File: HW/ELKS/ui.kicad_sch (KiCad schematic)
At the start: 29 parts, among them SW1 SW, SW2 SW, SW3 SW

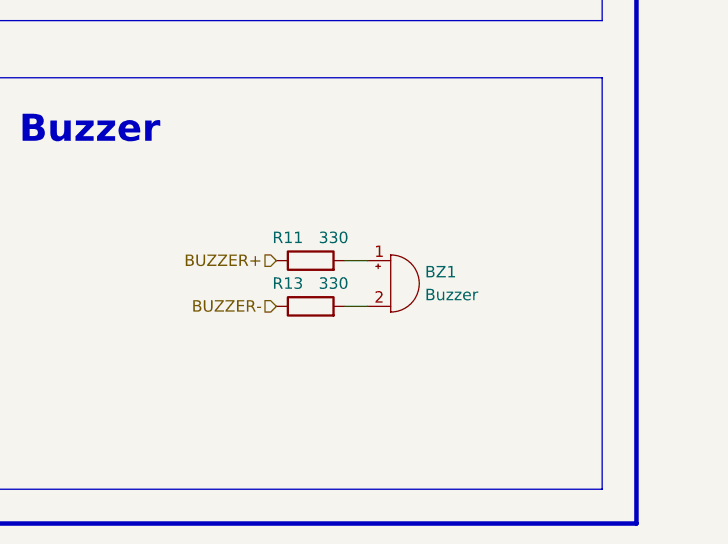
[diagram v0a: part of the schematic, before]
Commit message: Cleaning files
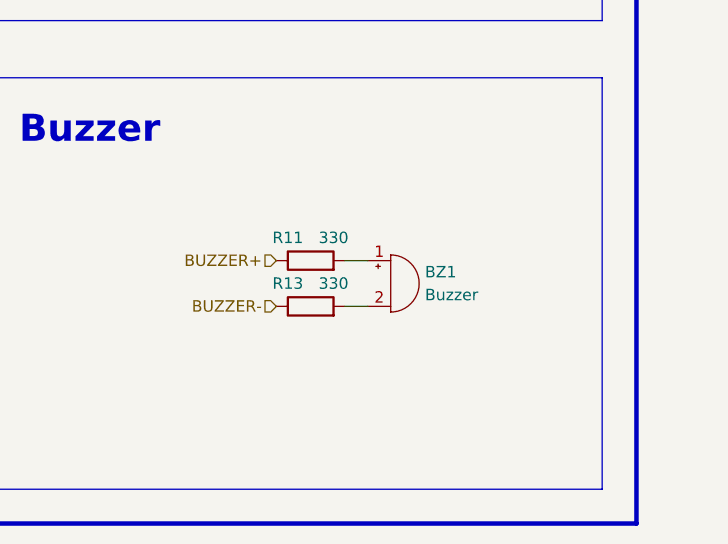
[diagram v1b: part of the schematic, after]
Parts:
- D3: LCSC C72043 -> C434423
